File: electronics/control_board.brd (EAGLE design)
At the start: 190 x 180 mm, 137 parts, among them J17 JST_PH_B3B-PH-K-S(LF)(SN), J18 JST_PH_B3B-PH-K-S(LF)(SN), J19 JST_PH_B3B-PH-K-S(LF)(SN), J20 JST_PH_B3B-PH-K-S(LF)(SN), J21 JST_PH_B3B-PH-K-S(LF)(SN), J22 JST_PH_B3B-PH-K-S(LF)(SN), J23 JST_PH_B3B-PH-K-S(LF)(SN), J24 JST_PH_B3B-PH-K-S(LF)(SN), J25 JST_PH_B3B-PH-K-S(LF)(SN), J26 JST_PH_B3B-PH-K-S(LF)(SN), J27 JST_PH_B3B-PH-K-S(LF)(SN), J28 JST_PH_B3B-PH-K-S(LF)(SN), J29 JST_PH_B3B-PH-K-S(LF)(SN), J30 JST_PH_B3B-PH-K-S(LF)(SN), J31 JST_PH_B3B-PH-K-S(LF)(SN), J32 JST_PH_B3B-PH-K-S(LF)(SN), U18 AD7730BRUZ, U19 AD5360BSTZ, U20 ADR425ARZ, U21 AD7730BRUZ, U23 AD7730BRUZ, U24 AD7730BRUZ, U25 AD7730BRUZ, U26 AD7730BRUZ, U27 AD7730BRUZ, U28 AD7730BRUZ, U4 ADR421ARZ, U5 AD7616BSTZ, X1 22-23-2031, Y1 KC2520B-C1, Y3 KC2520B-C1

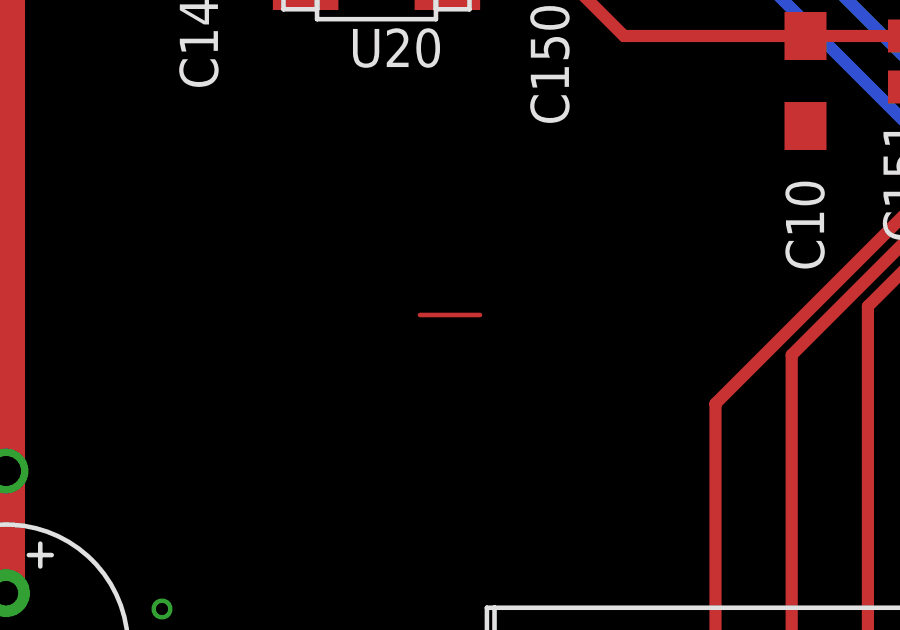
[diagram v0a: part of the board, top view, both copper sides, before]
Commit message: teensy test v0.0
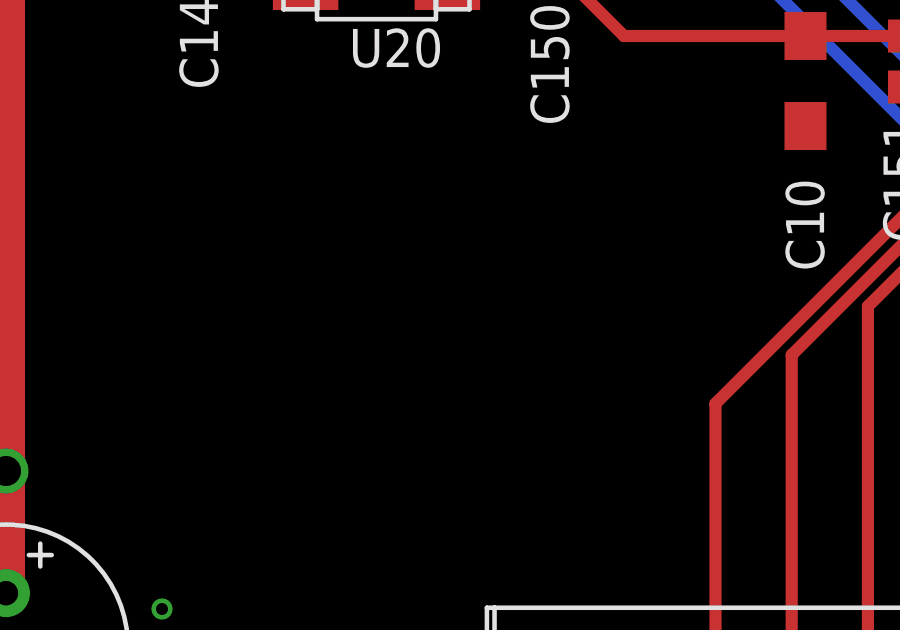
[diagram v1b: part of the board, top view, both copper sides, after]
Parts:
- R1, R3: value 68 -> 120
- R10: value 680 -> 1k
- R11: value 330 -> 120
- R5: value 220 -> 330
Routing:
- net N$1: track 2.00 -> 0.00 mm
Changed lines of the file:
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@@
 <attribute name="VALUE" x="7.305" y="172.272" size="1.27" layer="51" align="center"/>
 </element>
-<element name="R1" library="resistor" library_urn="urn:adsk.eagle:library:348" package="R0805" package3d_urn="urn:adsk.eagle:package:26059/1" value="68" x="160.55" y="166.4" smashed="yes" rot="R270">
+<element name="R1" library="resistor" library_urn="urn:adsk.eagle:library:348" package="R0805" package3d_urn="urn:adsk.eagle:package:26059/1" value="120" x="160.55" y="166.4" smashed="yes" rot="R270">
 <attribute name="NAME" x="159.87" y="164.135" size="1.27" layer="25" rot="R270"/>
 <attribute name="VALUE" x="158.01" y="167.035" size="1.27" layer="27" rot="R270"/>
 </element>
-<element name="R3" library="resistor" library_urn="urn:adsk.eagle:library:348" package="R0805" package3d_urn="urn:adsk.eagle:package:26059/1" value="68" x="154.7" y="166.4" smashed="yes" rot="R270">
+<element name="R3" library="resistor" library_urn="urn:adsk.eagle:library:348" package="R0805" package3d_urn="urn:adsk.eagle:package:26059/1" value="120" x="154.7" y="166.4" smashed="yes" rot="R270">
 <attribute name="NAME" x="154.02" y="164.085" size="1.27" layer="25" rot="R270"/>
 <attribute name="VALUE" x="152.16" y="167.035" size="1.27" layer="27" rot="R270"/>
 </element>
-<element name="R5" library="resistor" library_urn="urn:adsk.eagle:library:348" package="R0805" package3d_urn="urn:adsk.eagle:package:26059/1" value="220" x="148.85" y="166.4" smashed="yes" rot="R270">
+<element name="R5" library="resistor" library_urn="urn:adsk.eagle:library:348" package="R0805" package3d_urn="urn:adsk.eagle:package:26059/1" value="330" x="148.85" y="166.4" smashed="yes" rot="R270">
 <attribute name="NAME" x="148.17" y="164.135" size="1.27" layer="25" rot="R270"/>
 <attribute name="VALUE" x="146.31" y="167.035" size="1.27" layer="27" rot="R270"/>
 </element>
-<element name="R10" library="resistor" library_urn="urn:adsk.eagle:library:348" package="R0805" package3d_urn="urn:adsk.eagle:package:26059/1" value="680" x="166.4" y="166.4" smashed="yes" rot="R270">
+<element name="R10" library="resistor" library_urn="urn:adsk.eagle:library:348" package="R0805" package3d_urn="urn:adsk.eagle:package:26059/1" value="1k" x="166.4" y="166.4" smashed="yes" rot="R270">
 <attribute name="NAME" x="165.77" y="164.135" size="1.27" layer="25" rot="R270"/>
 <attribute name="VALUE" x="163.86" y="167.035" size="1.27" layer="27" rot="R270"/>
@@
 <attribute name="VALUE" x="-8.33" y="157.21" size="1.27" layer="27" ratio="10" rot="R270"/>
 </element>
-<element name="R11" library="resistor" library_urn="urn:adsk.eagle:library:348" package="R0805" package3d_urn="urn:adsk.eagle:package:26059/1" value="330" x="17.6" y="141.05" smashed="yes">
+<element name="R11" library="resistor" library_urn="urn:adsk.eagle:library:348" package="R0805" package3d_urn="urn:adsk.eagle:package:26059/1" value="120" x="17.6" y="141.05" smashed="yes">
 <attribute name="NAME" x="16.315" y="142.32" size="1.27" layer="25"/>
 <attribute name="VALUE" x="16.965" y="138.51" size="1.27" layer="27"/>
@@
 <wire x1="4.072" y1="146.9" x2="0.45" y2="146.9" width="1.016" layer="1"/>
 </signal>
-<signal name="N$1">
-<wire x1="110" y1="38.35" x2="112" y2="38.35" width="0.1524" layer="1"/>
-</signal>
 </signals>
